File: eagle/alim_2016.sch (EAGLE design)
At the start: 74 parts, among them J1 AVR_SPI_PRG_6PTH, U1 3.3V, U4 LM2596S-ADJ, U6 ATMEGA328P_TQFP

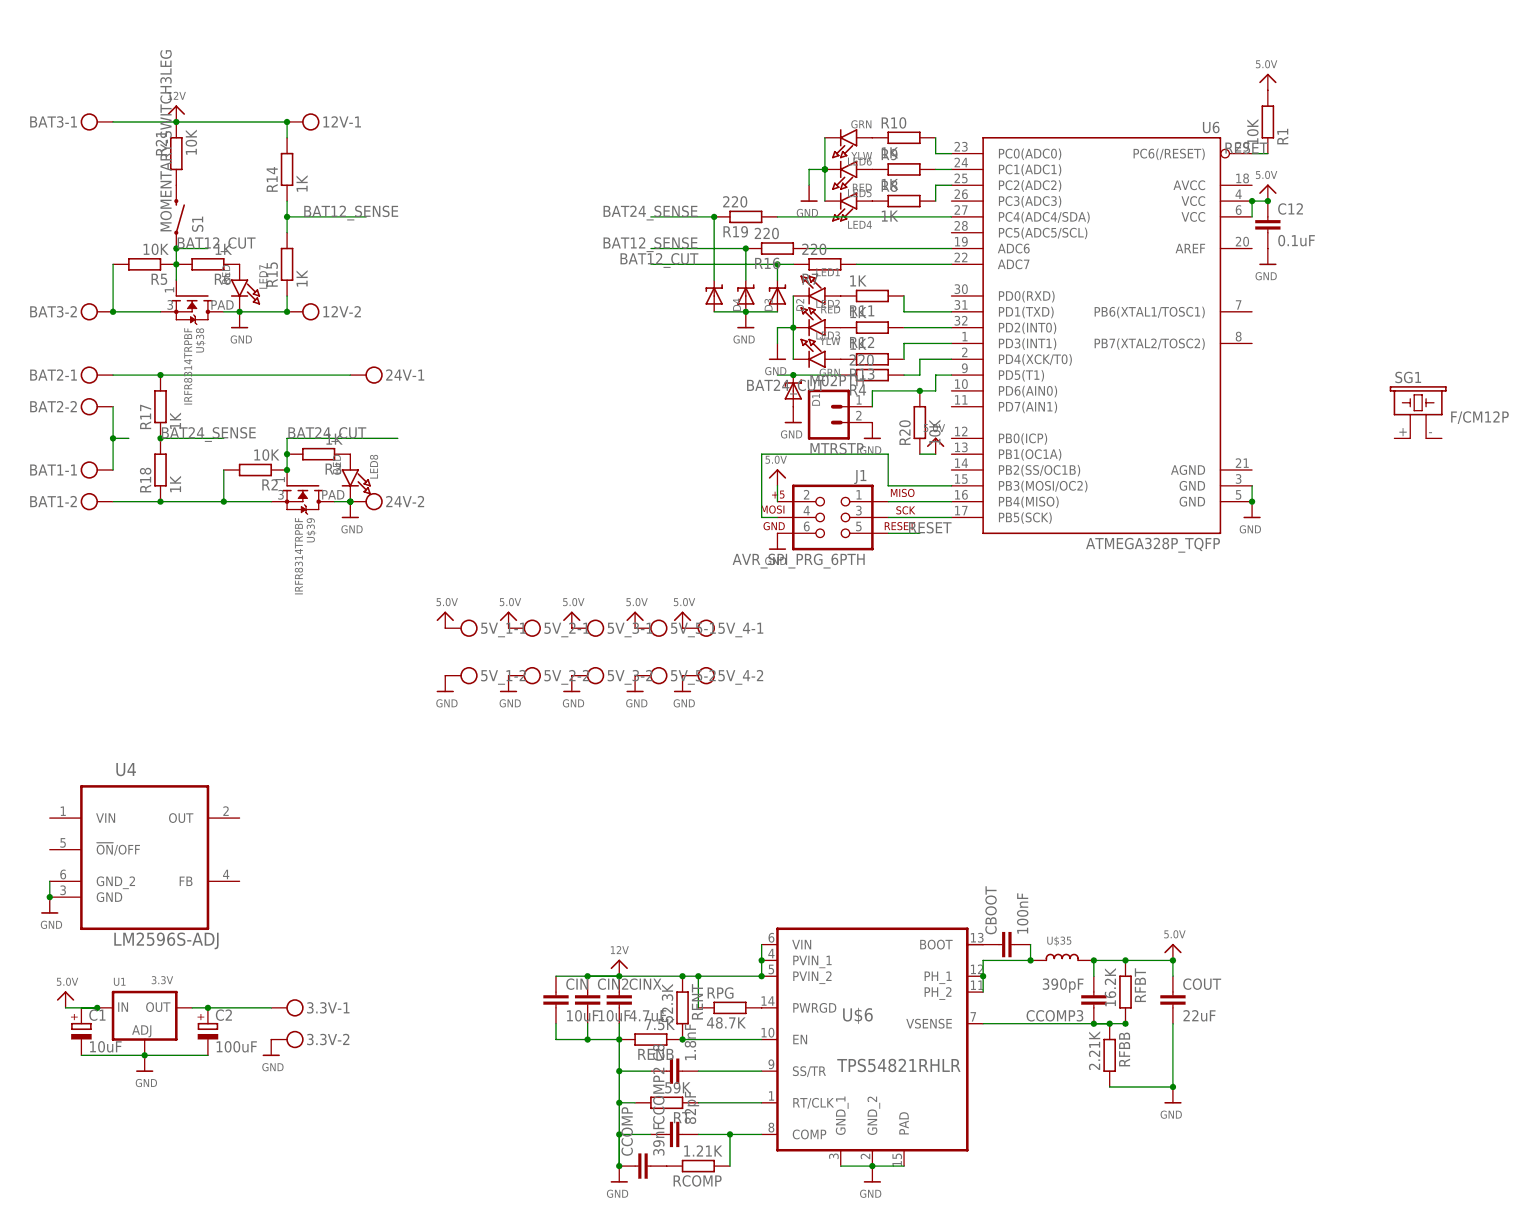
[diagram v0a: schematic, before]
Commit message: final version
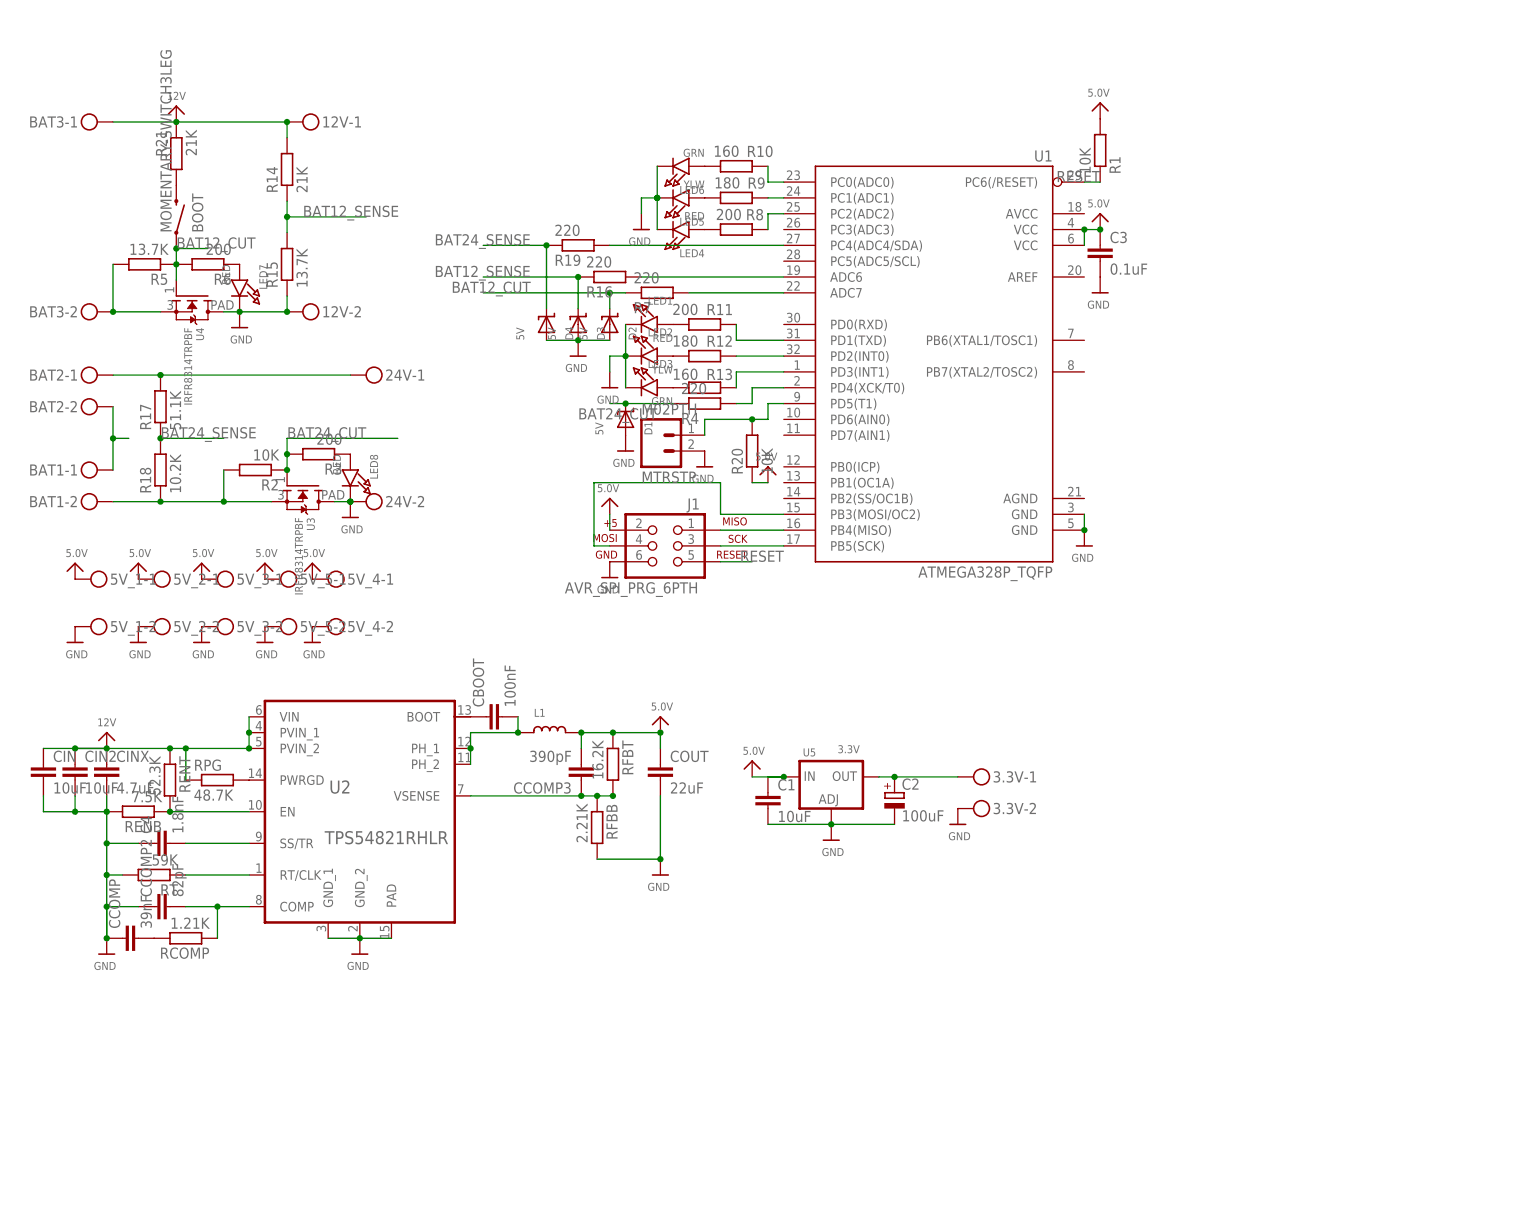
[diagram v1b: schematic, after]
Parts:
- removed C12: 0.1uF, rcl:C-EUC0805
- removed C8: 1.8nF, rcl:C-EUC0805
- removed SG1: F/CM12P, buzzer:F/CM12P
- removed U$35: 2.2uH, alim:XAL5030
- removed U$38: IRFR8314TRPBF, alim:IRFR8314TRPBF
- removed U$6: TPS54821RHLR, alim:TPS54821RHLR
- removed U6: ATMEGA328P_TQFP, SparkFun-DigitalIC:ATMEGA328P_TQFP
- added C3: 0.1uF, rcl:C-EUC0805
- added C4: 1.8nF, rcl:C-EUC0805
- added L1: 2.2uH, alim:XAL5030
- added U2: TPS54821RHLR, alim:TPS54821RHLR
- added U5: 3.3V, microbuilder:LM1117TO252
- C1: device rcl:CPOL-EUE2.5-7 -> rcl:C-EUC0805
- D1, D2, D3, D4: value (none) -> 5V
- R10, R13: value 1K -> 160
- R11, R3, R6, R8: value 1K -> 200
- R12, R9: value 1K -> 180
- R14: value 1K -> 21K
- R15: value 1K -> 13.7K
- R17: value 1K -> 51.1K
- R18: value 1K -> 10.2K
- R21: value 10K -> 21K
- R5: value 10K -> 13.7K
- U1: value 3.3V -> ATMEGA328P_TQFP; device microbuilder:LM1117TO252 -> SparkFun-DigitalIC:ATMEGA328P_TQFP
- U4: value LM2596S-ADJ -> IRFR8314TRPBF; device alim:LM2596S-ADJ -> alim:IRFR8314TRPBF
- renumbered S1 to BOOT, U$39 to U3
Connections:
- net 12V: now also U2.PVIN_1, U2.PVIN_2, U2.VIN; no longer U$6.PVIN_1, U$6.PVIN_2, U$6.VIN
- net 5.0V: now also C1.1, C3.1, L1.2, U1.VCC@4, U1.VCC@6, U5.IN; no longer C1.+, C12.1, U$35.2, U1.IN, U6.VCC@4, U6.VCC@6
- net BAT12_CUT: now also U4.G; no longer U$38.G
- net COMP: now also U2.COMP; no longer U$6.COMP
- net EN: now also U2.EN; no longer U$6.EN
- net GND: now also C1.2, C3.2, C4.1, U1.GND@3, U1.GND@5, U2.GND_1, U2.GND_2, U2.PAD, U4.D, U5.ADJ; no longer C1.-, C12.2, C8.1, U$38.D, U$6.GND_1, U$6.GND_2, U$6.PAD, U1.ADJ, U4.GND, U4.GND_2, U6.GND@3, U6.GND@5
- net N$1: now also U5.OUT; no longer U1.OUT
- net N$11: now also U1.PD4(XCK/T0); no longer U6.PD4(XCK/T0)
- net N$13: now also U4.S; no longer U$38.S
- net N$14: now also U1.PC1(ADC1); no longer U6.PC1(ADC1)
- net N$2: now also U1.PB5(SCK); no longer U6.PB5(SCK)
- net N$21: now also U1.PC2(ADC2); no longer U6.PC2(ADC2)
- net N$22: now also U1.PC0(ADC0); no longer U6.PC0(ADC0)
- net N$23: now also U1.ADC7; no longer U6.ADC7
- net N$24: now also U1.PD3(INT1); no longer U6.PD3(INT1)
- net N$25: now also U1.PD2(INT0); no longer U6.PD2(INT0)
- net N$26: now also U1.PD1(TXD); no longer U6.PD1(TXD)
- net N$27: now also U1.ADC6; no longer U6.ADC6
- net N$28: now also U1.PC4(ADC4/SDA); no longer U6.PC4(ADC4/SDA)
- net N$3: now also U1.PB4(MISO); no longer U6.PB4(MISO)
- net N$31: now also U2.BOOT; no longer U$6.BOOT
- net N$35: now also U2.PWRGD; no longer U$6.PWRGD
- net N$4: now also U1.PB3(MOSI/OC2); no longer U6.PB3(MOSI/OC2)
- net N$6: now also U1.PD5(T1); no longer U6.PD5(T1)
- net PH: now also L1.1, U2.PH_1, U2.PH_2; no longer U$35.1, U$6.PH_1, U$6.PH_2
- net RESET: now also U1.PC6(/RESET); no longer U6.PC6(/RESET)
- net RTCLK: now also U2.RT/CLK; no longer U$6.RT/CLK
- net SSTR: now also C4.2, U2.SS/TR; no longer C8.2, U$6.SS/TR
- net VSENSE: now also U2.VSENSE; no longer U$6.VSENSE
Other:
- moved on the sheet: 3.3V-1, 3.3V-2, 5V_1-1, 5V_1-2, 5V_2-1, 5V_2-2, 5V_3-1, 5V_3-2, 5V_4-1, 5V_4-2, 5V_5-1, 5V_5-2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
